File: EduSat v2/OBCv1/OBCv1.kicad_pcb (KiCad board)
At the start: 2 copper layers, 80.5 x 80.5 mm, 10 parts, among them J1 Conn_02x20_Odd_Even, J2 USB_C_Receptacle_USB2.0_16P, U1 ESP32-WROOM-32E, U2 CP2102N-Axx-xQFN28, U3 Ai-Thinker-Ra-02

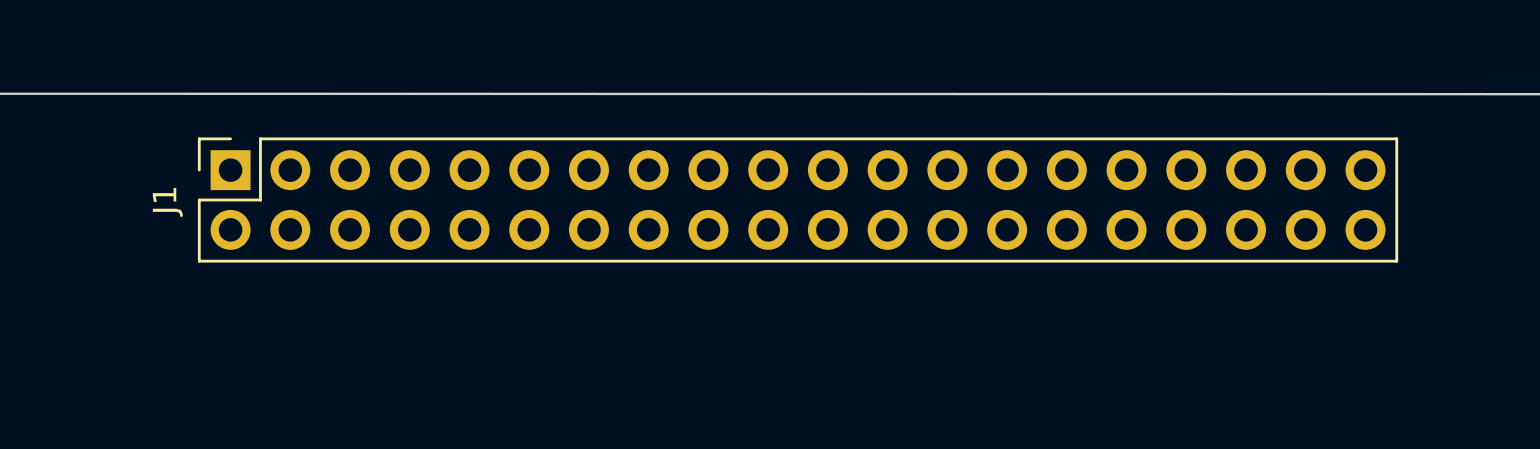
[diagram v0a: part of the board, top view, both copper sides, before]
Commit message: More updates
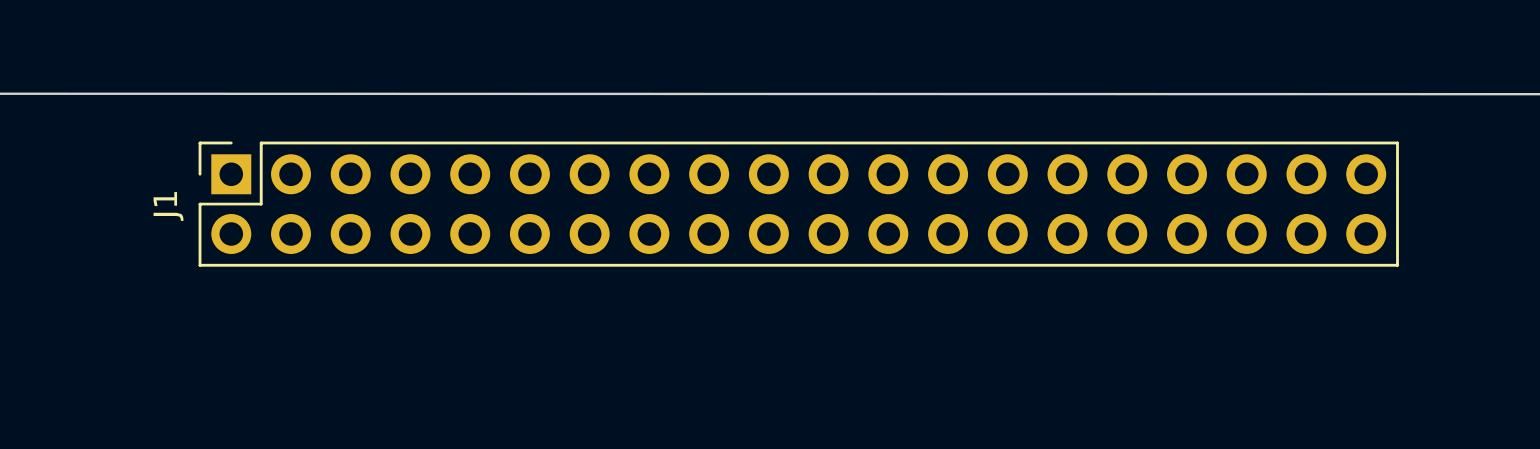
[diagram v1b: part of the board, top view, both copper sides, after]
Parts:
- moved J1 0.18 mm to (67.0, 49.9)
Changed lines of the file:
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@@
 		(allow_soldermask_bridges_in_footprints no)
 		(aux_axis_origin 50.8 127)
-		(grid_origin 50.8 127)
+		(grid_origin 91.070259 86.735491)
 		(pcbplotparams
 			(layerselection 0x00010fc_ffffffff)
@@
 		(tags "USB C Type-C Receptacle SMD")
 		(property "Reference" "J2"
-			(at 0 -5.715 270)
+			(at 0 -5.715 -90)
 			(layer "F.SilkS")
 			(effects
@@
 		)
 		(fp_text user "${REFERENCE}"
-			(at 0 0 270)
+			(at 0 0 -90)
 			(layer "F.Fab")
 			(effects
@@
 		(locked yes)
 		(layer "F.Cu")
-		(at 66.940388 49.710258 90)
+		(at 66.970259 49.885491 90)
 		(descr "Through hole straight socket strip, 2x20, 2.54mm pitch, double cols (from Kicad 4.0.7), script generated")
 		(tags "Through hole socket strip THT 2x20 2.54mm double row")
 		(property "Reference" "J1"
-			(at -1.27 -2.77 270)
+			(at -1.27 -2.77 -90)
 			(layer "F.SilkS")
 			(effects
@@
 		)
 		(fp_text user "${REFERENCE}"
-			(at -1.27 24.13 360)
+			(at -1.27 24.13 0)
 			(layer "F.Fab")
 			(effects
@@
 		(tags "LoRa Ra-01")
 		(property "Reference" "U3"
-			(at 0 -1 270)
+			(at 0 -1 -90)
 			(layer "F.SilkS")
 			(effects
@@
 		)
 		(property "Value" "Ai-Thinker-Ra-02"
-			(at 0 9.75 270)
+			(at 0 9.75 -90)
 			(layer "F.Fab")
 			(effects
@@
 		)
 		(fp_text user "${REFERENCE}"
-			(at 0 1 270)
+			(at 0 1 -90)
 			(layer "F.Fab")
 			(effects
@@
 			)
 			(layer "F.Fab")
-			(net 7471205)
 		)
 		(fp_line
@@
 			)
 			(layer "F.Fab")
-			(net 7471205)
 		)
 		(fp_line
@@
 			)
 			(layer "F.Fab")
-			(net 7471205)
 		)
 		(fp_line
@@
 			)
 			(layer "F.Fab")
-			(net 7471205)
 		)
 		(fp_line
@@
 			)
 			(layer "F.Fab")
-			(net 7471205)
 		)
 		(fp_line
@@
 			)
 			(layer "F.Fab")
-			(net 7471205)
 		)
 		(fp_line
@@
 			)
 			(layer "F.Fab")
-			(net 7471205)
 		)
 		(fp_line
@@
 			)
 			(layer "F.Fab")
-			(net 7471205)
 		)
 		(fp_line
@@
 			)
 			(layer "F.Fab")
-			(net 7471205)
 		)
 		(fp_line
@@
 			)
 			(layer "F.Fab")
-			(net 7471205)
 		)
 		(fp_line
@@
 			)
 			(layer "F.Fab")
-			(net 7471205)
 		)
 		(fp_line
@@
 			)
 			(layer "F.Fab")
-			(net 7471205)
 		)
 		(fp_line
@@
 			)
 			(layer "F.Fab")
-			(net 7471205)
 		)
 		(fp_line
@@
 			)
 			(layer "F.Fab")
-			(net 7471205)
 		)
 		(fp_line
@@
 			)
 			(layer "F.Fab")
-			(net 7471205)
 		)
 		(fp_text user "Antenna"
@@
 		(start 50.801388 49.710258)
 		(end 50.8 123.75)
+		(locked yes)
 		(stroke
 			(width 0.1)
@@
 		(mid 51.751903 126.048097)
 		(end 50.8 123.75)
+		(locked yes)
 		(stroke
 			(width 0.1)
@@
 		(mid 51.753291 47.412161)
 		(end 54.051388 46.460258)
+		(locked yes)
 		(stroke
 			(width 0.1)
@@
 		(start 131.339824 49.732)
 		(end 131.339824 123.749705)
+		(locked yes)
 		(stroke
 			(width 0.1)
@@
 		(mid 130.387921 126.047802)
 		(end 128.089824 126.999705)
+		(locked yes)
 		(stroke
 			(width 0.1)
@@
 		(start 128.089824 126.999705)
 		(end 54.05 127)
+		(locked yes)
 		(stroke
 			(width 0.1)
@@
 		(start 54.051388 46.460258)
 		(end 128.089824 46.482)
+		(locked yes)
 		(stroke
 			(width 0.1)
@@
 		(mid 130.387921 47.433903)
 		(end 131.339824 49.732)
+		(locked yes)
 		(stroke
 			(width 0.1)
